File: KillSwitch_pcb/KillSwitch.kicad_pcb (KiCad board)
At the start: 2 copper layers, 97.8 x 69.8 mm, 82 parts, among them IC1 Wio-SX1262, J1 J_ESP_DBG_UART, J2 USB_C_Receptacle_USB2.0, SW1 SW_DIP_x08, SW2 SW_RESET, SW4 ARM, SW5 KILL1, SW6 KILL2, SW7 KILL3, SW8 KILL4, SW9 SW_BATT, U1 ESP32-S3-WROOM-1, U2 MCP23017_SO, U3 MCP101-315D, U4 AP7361C-33E, U5 AP7361C-33E

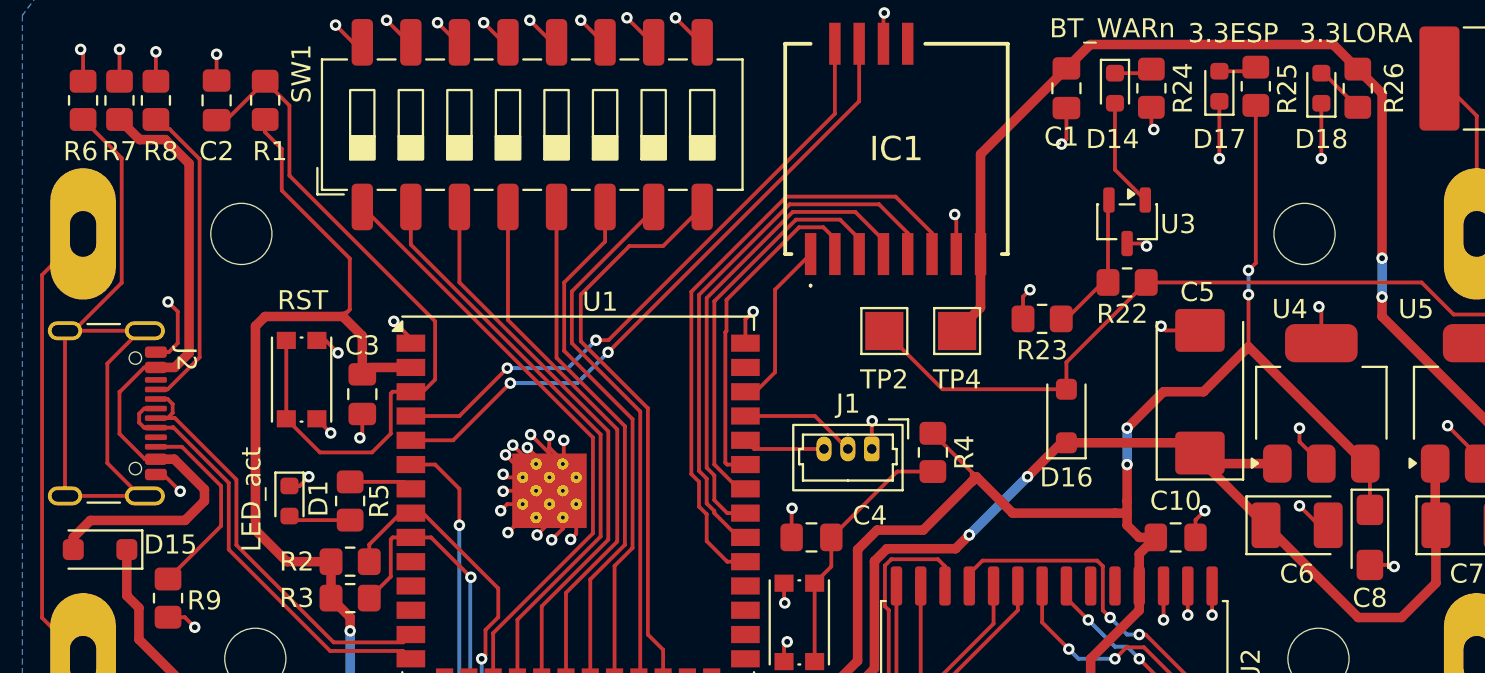
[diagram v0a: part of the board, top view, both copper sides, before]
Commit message: mini poprawki
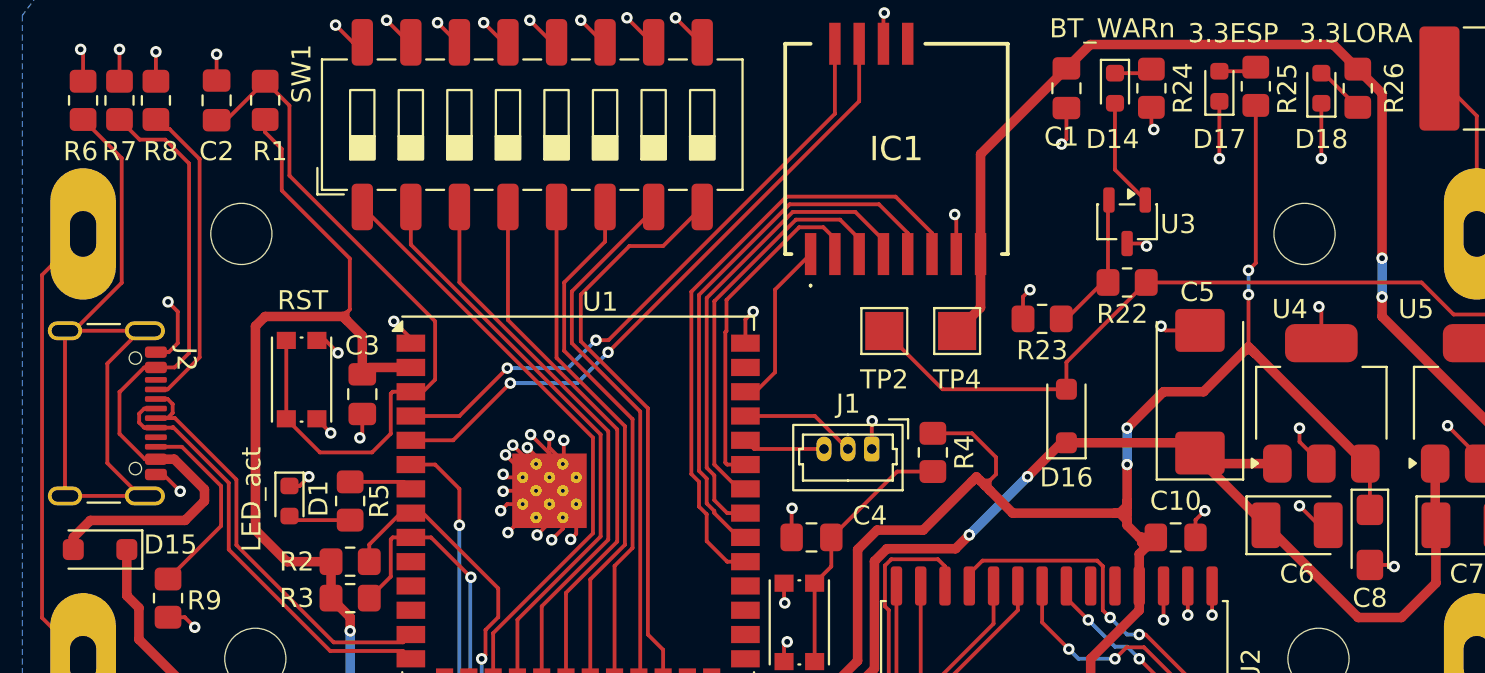
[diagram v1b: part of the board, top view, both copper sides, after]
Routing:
- net /+3.3v_ESP: track 152.0 -> 157.6 mm
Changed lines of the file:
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@@
+	)
+	(segment
+		(start 186.944 71.755)
+		(end 187.325 71.374)
+		(width 0.5)
+		(layer "F.Cu")
+		(net 6)
 	)
 	(segment
@@
 	)
 	(segment
-		(start 179.197 69.723)
-		(end 179.197 70.104)
-		(width 0.2)
+		(start 146.4945 61.6585)
+		(end 146.304 61.468)
+		(width 0.5)
+		(layer "F.Cu")
+		(net 6)
+	)
+	(segment
+		(start 179.443 69.858)
+		(end 179.6335 70.0485)
+		(width 0.5)
+		(layer "F.Cu")
+		(net 6)
+	)
+	(segment
+		(start 193.516 63.214)
+		(end 193.675 63.055)
+		(width 0.5)
 		(layer "F.Cu")
 		(net 6)
@@
 	)
 	(segment
+		(start 179.213 67.58)
+		(end 180.467 68.834)
+		(width 0.2)
+		(layer "F.Cu")
+		(net 6)
+	)
+	(segment
 		(start 194.056 50.4285)
 		(end 194.056 58.674)
@@
 	(segment
 		(start 187.325 71.755)
-		(end 187.325 71.12)
-		(width 0.5)
+		(end 187.325 71.374)
+		(width 0.5)
+		(layer "F.Cu")
+		(net 6)
+	)
+	(segment
+		(start 188.33025 73.52225)
+		(end 187.96 73.8925)
+		(width 0.5)
+		(layer "F.Cu")
+		(net 6)
+	)
+	(segment
+		(start 180.1415 70.0485)
+		(end 179.6335 70.0485)
+		(width 0.2)
 		(layer "F.Cu")
 		(net 6)
@@
 	)
 	(segment
+		(start 177.165 67.58)
+		(end 179.213 67.58)
+		(width 0.2)
+		(layer "F.Cu")
+		(net 6)
+	)
+	(segment
 		(start 145.685 74.295)
 		(end 145.685 76.2)
@@
 	)
 	(segment
-		(start 179.443 69.858)
-		(end 181.34 71.755)
-		(width 0.5)
-		(layer "F.Cu")
-		(net 6)
-	)
-	(segment
-		(start 179.2525 69.6675)
-		(end 179.197 69.723)
-		(width 0.2)
+		(start 179.8875 70.3025)
+		(end 180.1415 70.5565)
+		(width 0.5)
+		(layer "F.Cu")
+		(net 6)
+	)
+	(segment
+		(start 186.944 71.755)
+		(end 187.325 71.755)
+		(width 0.5)
 		(layer "F.Cu")
 		(net 6)
@@
 	)
 	(segment
+		(start 193.834 63.214)
+		(end 193.516 63.214)
+		(width 0.5)
+		(layer "F.Cu")
+		(net 6)
+	)
+	(segment
 		(start 147.32 81.28)
 		(end 146.685 80.645)
@@
 	)
 	(segment
+		(start 187.325 72.136)
+		(end 187.325 71.755)
+		(width 0.5)
+		(layer "F.Cu")
+		(net 6)
+	)
+	(segment
 		(start 173.228 73.66)
 		(end 173.228 79.484768)
@@
 	)
 	(segment
+		(start 194.0245 63.4045)
+		(end 193.675 63.055)
+		(width 0.5)
+		(layer "F.Cu")
+		(net 6)
+	)
+	(segment
 		(start 200.025 69.405)
 		(end 199.785 69.165)
@@
 	(segment
 		(start 188.8275 73.025)
-		(end 187.96 73.8925)
+		(end 188.33025 73.52225)
+		(width 0.5)
+		(layer "F.Cu")
+		(net 6)
+	)
+	(segment
+		(start 194.0245 63.4045)
+		(end 193.834 63.214)
 		(width 0.5)
 		(layer "F.Cu")
@@
 	)
 	(segment
+		(start 180.1495 70.0405)
+		(end 179.8875 70.3025)
+		(width 0.2)
+		(layer "F.Cu")
+		(net 6)
+	)
+	(segment
+		(start 146.558 61.214)
+		(end 146.558 61.595)
+		(width 0.2)
+		(layer "F.Cu")
+		(net 6)
+	)
+	(segment
 		(start 146.66745 61.10455)
 		(end 146.304 61.468)
@@
 	)
 	(segment
+		(start 180.1495 70.0405)
+		(end 180.1415 70.0485)
+		(width 0.2)
+		(layer "F.Cu")
+		(net 6)
+	)
+	(segment
+		(start 180.467 69.723)
+		(end 180.1495 70.0405)
+		(width 0.2)
+		(layer "F.Cu")
+		(net 6)
+	)
+	(segment
 		(start 142.2025 51.2025)
 		(end 142.24 51.165)
@@
 	)
 	(segment
-		(start 179.2525 69.6675)
-		(end 179.443 69.858)
+		(start 186.944 71.755)
+		(end 187.325 72.136)
+		(width 0.5)
+		(layer "F.Cu")
+		(net 6)
+	)
+	(segment
+		(start 180.1415 70.5565)
+		(end 181.34 71.755)
+		(width 0.5)
+		(layer "F.Cu")
+		(net 6)
+	)
+	(segment
+		(start 146.558 61.595)
+		(end 146.4945 61.6585)
 		(width 0.2)
 		(layer "F.Cu")
@@
 	(segment
 		(start 188.8275 73.025)
-		(end 187.96 73.025)
+		(end 188.087 73.025)
 		(width 0.5)
 		(layer "F.Cu")
@@
 	(segment
 		(start 187.325 72.39)
-		(end 187.325 71.755)
+		(end 187.325 72.136)
 		(width 0.5)
 		(layer "F.Cu")
@@
 	(segment
 		(start 199.785 69.165)
-		(end 193.675 63.055)
+		(end 194.0245 63.4045)
 		(width 0.5)
 		(layer "F.Cu")
@@
 	)
 	(segment
+		(start 188.087 73.279)
+		(end 188.087 73.025)
+		(width 0.5)
+		(layer "F.Cu")
+		(net 6)
+	)
+	(segment
 		(start 193.675 63.055)
 		(end 193.675 62.865)
@@
 	)
 	(segment
+		(start 188.087 73.025)
+		(end 187.96 73.025)
+		(width 0.5)
+		(layer "F.Cu")
+		(net 6)
+	)
+	(segment
+		(start 180.467 68.834)
+		(end 180.467 69.723)
+		(width 0.2)
+		(layer "F.Cu")
+		(net 6)
+	)
+	(segment
 		(start 181.34 71.755)
 		(end 186.69 71.755)
@@
 	)
 	(segment
+		(start 180.1415 70.0485)
+		(end 180.1415 70.5565)
+		(width 0.2)
+		(layer "F.Cu")
+		(net 6)
+	)
+	(segment
 		(start 187.96 73.8925)
 		(end 187.96 75.565)
@@
 	)
 	(segment
-		(start 177.165 67.58)
-		(end 179.2525 69.6675)
-		(width 0.2)
+		(start 187.325 71.374)
+		(end 187.325 71.12)
+		(width 0.5)
 		(layer "F.Cu")
 		(net 6)
@@
 	(segment
 		(start 186.69 71.755)
-		(end 187.325 71.755)
+		(end 186.944 71.755)
 		(width 0.5)
 		(layer "F.Cu")
@@
 	(segment
 		(start 147.32 62.484)
-		(end 146.304 61.468)
+		(end 146.4945 61.6585)
 		(width 0.5)
 		(layer "F.Cu")
@@
 	(segment
 		(start 191.325 65.405)
-		(end 193.675 63.055)
+		(end 193.516 63.214)
 		(width 0.5)
 		(layer "F.Cu")
@@
 	)
 	(segment
+		(start 179.6335 70.0485)
+		(end 179.8875 70.3025)
+		(width 0.5)
+		(layer "F.Cu")
+		(net 6)
+	)
+	(segment
+		(start 188.33025 73.52225)
+		(end 188.087 73.279)
+		(width 0.5)
+		(layer "F.Cu")
+		(net 6)
+	)
+	(segment
 		(start 147.447 82.042)
 		(end 147.32 81.915)
@@
 		(start 134.62 51.165)
 		(end 135.67355 52.21855)
-		(width 0.5)
+		(width 0.2)
 		(layer "F.Cu")
 		(net 36)
@@
 		(start 138.26 53.4671)
 		(end 138.26 63.379592)
-		(width 0.5)
+		(width 0.2)
 		(layer "F.Cu")
 		(net 36)
@@
 		(start 137.01145 52.21855)
 		(end 138.26 53.4671)
-		(width 0.5)
+		(width 0.2)
 		(layer "F.Cu")
 		(net 36)
@@
 		(start 138.26 63.379592)
 		(end 137.504592 64.135)
-		(width 0.5)
+		(width 0.2)
 		(layer "F.Cu")
 		(net 36)
@@
 		(start 135.67355 52.21855)
 		(end 137.01145 52.21855)
-		(width 0.5)
+		(width 0.2)
 		(layer "F.Cu")
 		(net 36)
@@
 		(start 137.504592 64.135)
 		(end 136.525 64.135)
-		(width 0.5)
+		(width 0.2)
 		(layer "F.Cu")
 		(net 36)
